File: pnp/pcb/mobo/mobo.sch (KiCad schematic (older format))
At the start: 19 parts, among them J5 Conn_ARM_JTAG_SWD_10, SW2 RESET, U1 STM32F407VETx, Y1 12MHz, Y3 32.768MHz

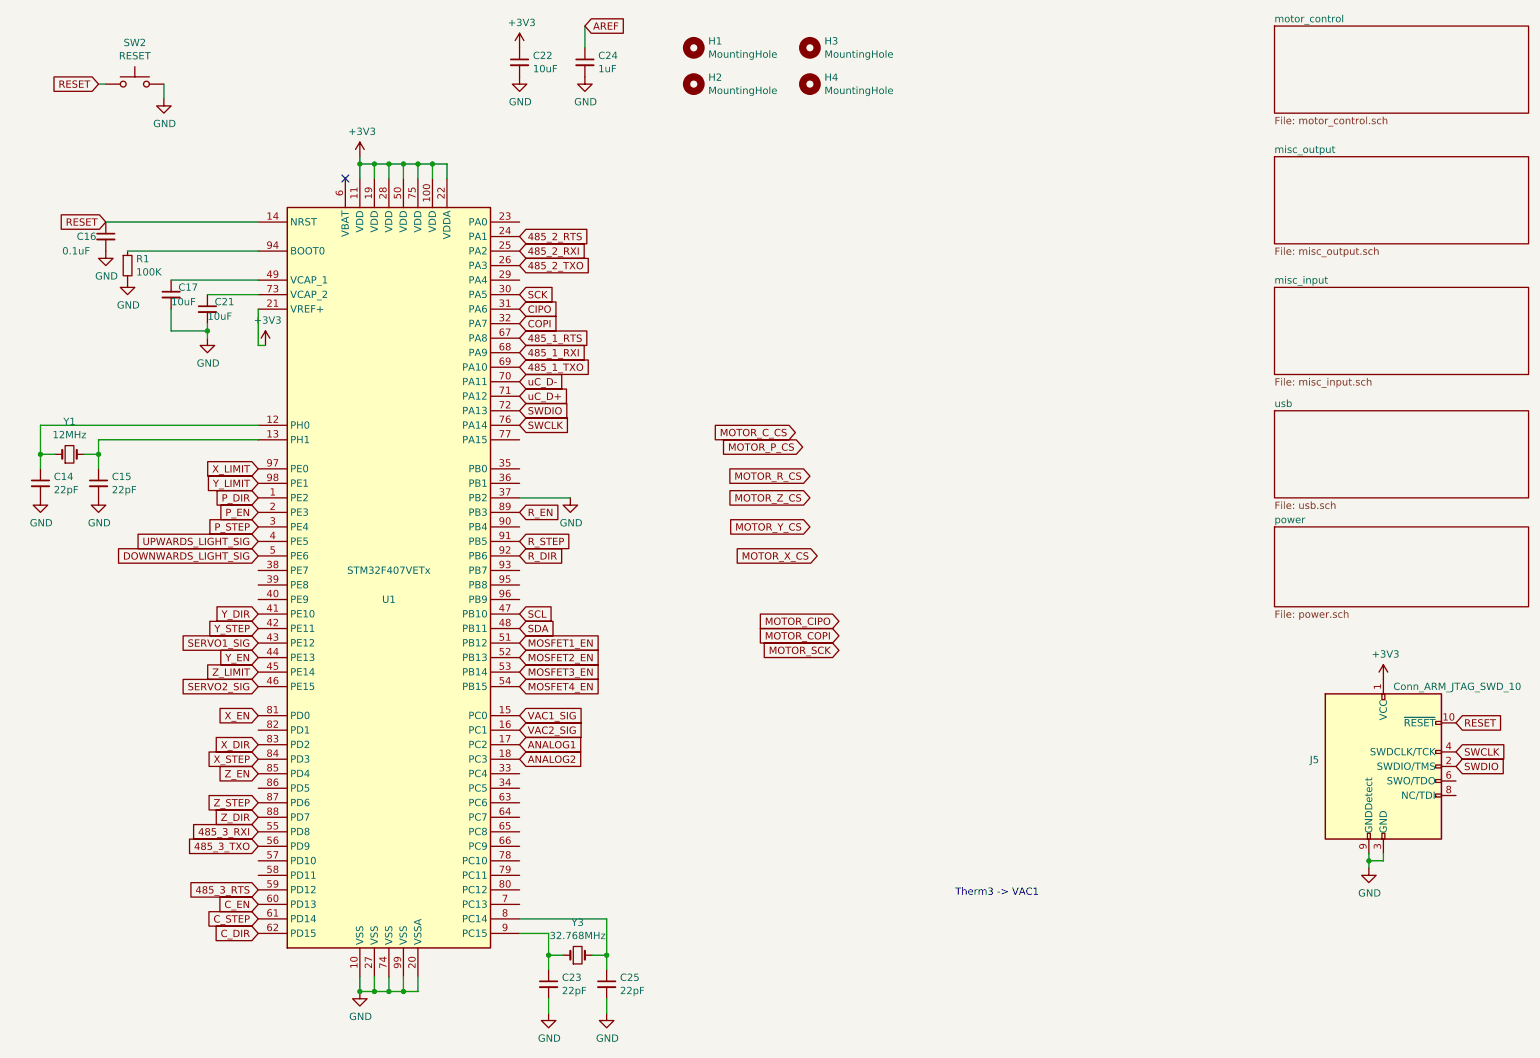
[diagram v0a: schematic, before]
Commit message: finished layout, going to try a different one, committing in case i mess it up
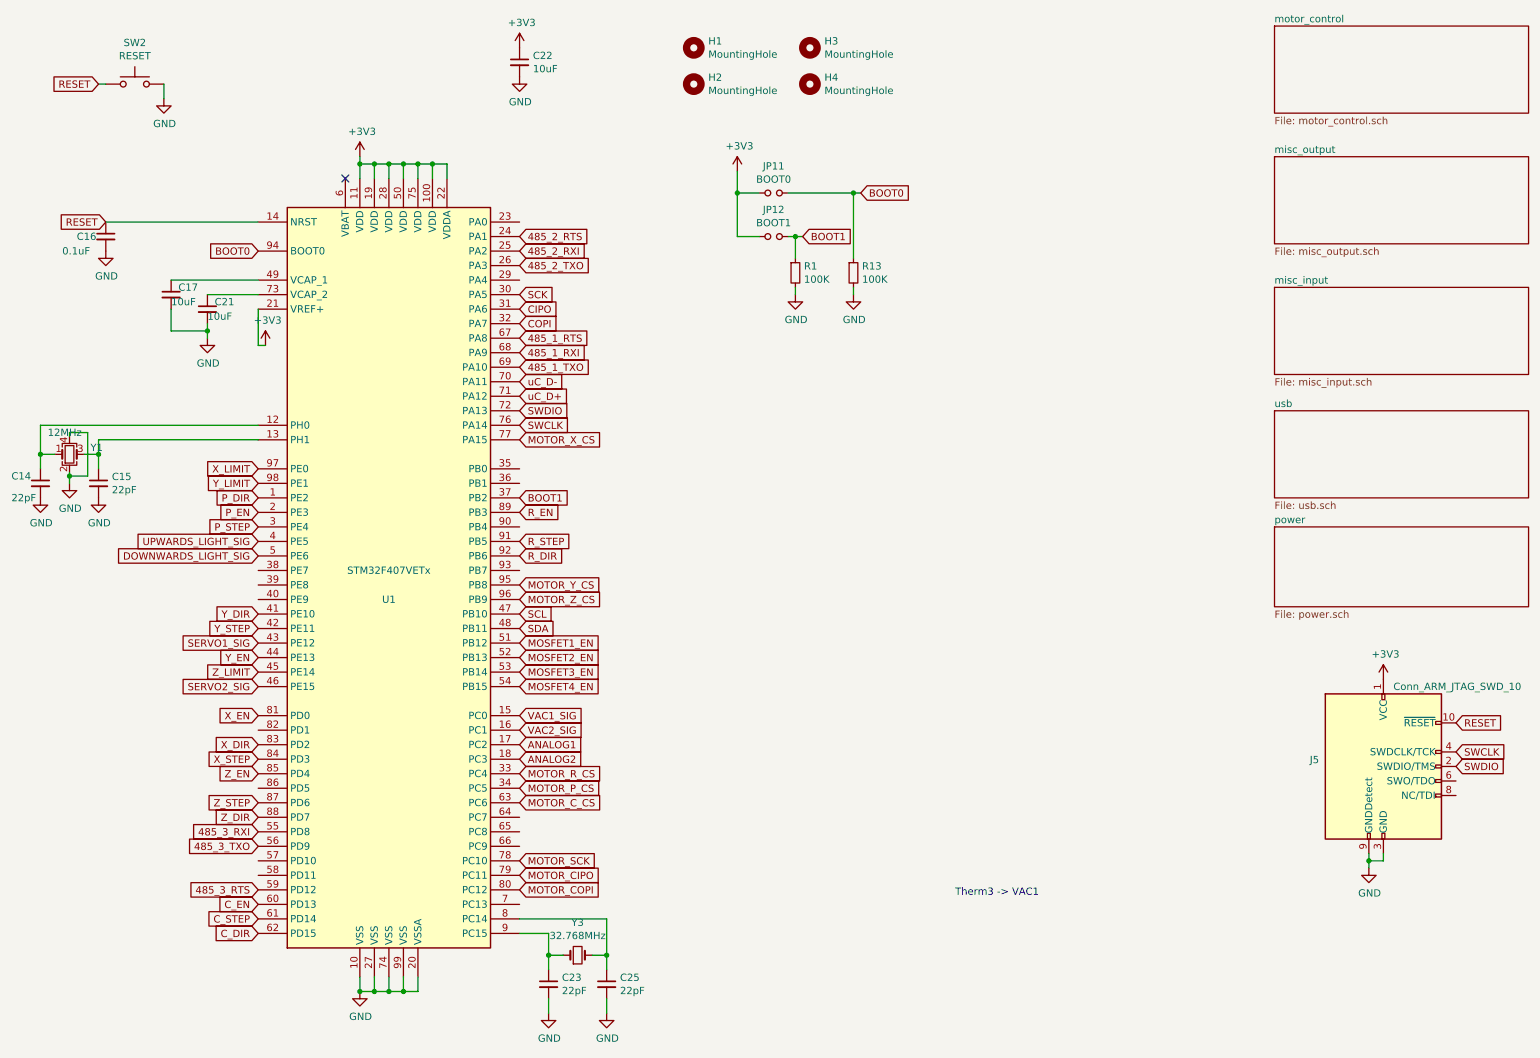
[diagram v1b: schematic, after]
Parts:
- removed C24: 1uF, Capacitor_SMD:C_0805_2012Metric_Pad1.15x1.40mm_HandSolder, symbol Device:C_Small
- removed Y1: 12MHz, Crystal:Crystal_SMD_0603-2Pin_6.0x3.5mm, symbol Device:Crystal_Small
- added JP11: BOOT0, Jumper:SolderJumper-2_P1.3mm_Open_RoundedPad1.0x1.5mm, symbol Device:Jumper_NO_Small
- added JP12: BOOT1, Jumper:SolderJumper-2_P1.3mm_Open_RoundedPad1.0x1.5mm, symbol Device:Jumper_NO_Small
- added R13: 100K, Resistor_SMD:R_0805_2012Metric_Pad1.15x1.40mm_HandSolder, symbol Device:R_Small
- added Y1: 12MHz, Crystal:Crystal_SMD_3225-4Pin_3.2x2.5mm, symbol Device:Crystal_GND24_Small
- Y3: footprint Crystal:Crystal_SMD_0603-2Pin_6.0x3.5mm -> Crystal:Crystal_SMD_3215-2Pin_3.2x1.5mm
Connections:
- net +3V3: now also JP11.1, JP12.1
- net GND: now also R13.2, Y1.2, Y1.4; no longer U1.37 (PB2)
- net MOTOR_CIPO: now also U1.79 (PC11)
- net MOTOR_COPI: now also U1.80 (PC12)
- net MOTOR_C_CS: now also U1.63 (PC6)
- net MOTOR_P_CS: now also U1.34 (PC5)
- net MOTOR_R_CS: now also U1.33 (PC4)
- net MOTOR_SCK: now also U1.78 (PC10)
- net MOTOR_X_CS: now also U1.77 (PA15)
- net MOTOR_Y_CS: now also U1.95 (PB8)
- net MOTOR_Z_CS: now also U1.96 (PB9)
- net at C14.1, U1.12 (PH0): now also Y1.1
- net at C15.1, U1.13 (PH1): now also Y1.3
- net BOOT0: now reaches U1.94 (BOOT0)
- net BOOT0: now also JP11.2, R13.1; no longer R1.1
- new net BOOT1: JP12.2, R1.1, U1.37 (PB2)
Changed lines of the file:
@@
 	1    0    0    -1
 $EndComp
-$Comp
-L Device:C_Small C24
-U 1 1 5EF034CB
-P 4450 900
-F 0 "C24" H 4542 946 50  0000 L CNN
-F 1 "1uF" H 4542 855 50  0000 L CNN
-F 2 "Capacitor_SMD:C_0805_2012Metric_Pad1.15x1.40mm_HandSolder" H 4450 900 50  0001 C CNN
-F 3 "~" H 4450 900 50  0001 C CNN
-	1    4450 900
-	1    0    0    -1
-$EndComp
-$Comp
-L power:GND #PWR0119
-U 1 1 5EF0394F
-P 4450 1000
-F 0 "#PWR0119" H 4450 750 50  0001 C CNN
-F 1 "GND" H 4455 827 50  0000 C CNN
-F 2 "" H 4450 1000 50  0001 C CNN
-F 3 "" H 4450 1000 50  0001 C CNN
-	1    4450 1000
-	1    0    0    -1
-$EndComp
-Text GLabel 4450 650  2    50   Input ~ 0
-AREF
-Wire Wire Line
-	4450 650  4450 800
 Connection ~ 2900 7300
 Wire Wire Line
@@
 $EndComp
 $Comp
-L Device:R_Small R1
-U 1 1 5F0D0BAB
-P 1300 2300
-F 0 "R1" H 1359 2346 50  0000 L CNN
-F 1 "100K" H 1359 2255 50  0000 L CNN
-F 2 "Resistor_SMD:R_0805_2012Metric_Pad1.15x1.40mm_HandSolder" H 1300 2300 50  0001 C CNN
-F 3 "~" H 1300 2300 50  0001 C CNN
-	1    1300 2300
-	1    0    0    -1
-$EndComp
-Wire Wire Line
-	1300 2200 2200 2200
-$Comp
-L power:GND #PWR0121
-U 1 1 5F0D3158
-P 1300 2400
-F 0 "#PWR0121" H 1300 2150 50  0001 C CNN
-F 1 "GND" H 1305 2227 50  0000 C CNN
-F 2 "" H 1300 2400 50  0001 C CNN
-F 3 "" H 1300 2400 50  0001 C CNN
-	1    1300 2400
-	1    0    0    -1
-$EndComp
-$Comp
 L Device:C_Small C17
 U 1 1 5F0D3862
@@
 	1850 2750 1850 2700
 $Comp
-L power:GND #PWR0123
-U 1 1 5F0DF8B3
-P 4350 3900
-F 0 "#PWR0123" H 4350 3650 50  0001 C CNN
-F 1 "GND" H 4355 3727 50  0000 C CNN
-F 2 "" H 4350 3900 50  0001 C CNN
-F 3 "" H 4350 3900 50  0001 C CNN
-	1    4350 3900
-	1    0    0    -1
-$EndComp
-Wire Wire Line
-	4000 3900 4350 3900
-$Comp
-L Device:Crystal_Small Y1
-U 1 1 5F0E1806
-P 900 3600
-F 0 "Y1" H 900 3825 50  0000 C CNN
-F 1 "12MHz" H 900 3734 50  0000 C CNN
-F 2 "Crystal:Crystal_SMD_0603-2Pin_6.0x3.5mm" H 900 3600 50  0001 C CNN
-F 3 "~" H 900 3600 50  0001 C CNN
-	1    900  3600
-	1    0    0    -1
-$EndComp
-$Comp
 L Device:Crystal_Small Y3
 U 1 1 5F0E266F
@@
 F 0 "Y3" H 4400 7275 50  0000 C CNN
 F 1 "32.768MHz" H 4400 7184 50  0000 C CNN
-F 2 "Crystal:Crystal_SMD_0603-2Pin_6.0x3.5mm" H 4400 7050 50  0001 C CNN
+F 2 "Crystal:Crystal_SMD_3215-2Pin_3.2x1.5mm" H 4400 7050 50  0001 C CNN
 F 3 "~" H 4400 7050 50  0001 C CNN
 	1    4400 7050
@@
 U 1 1 5F10974E
 P 700 3800
-F 0 "C14" H 792 3846 50  0000 L CNN
-F 1 "22pF" H 792 3755 50  0000 L CNN
+F 0 "C14" H 500 3850 50  0000 L CNN
+F 1 "22pF" H 500 3700 50  0000 L CNN
 F 2 "Capacitor_SMD:C_0805_2012Metric_Pad1.15x1.40mm_HandSolder" H 700 3800 50  0001 C CNN
 F 3 "~" H 700 3800 50  0001 C CNN
@@
 Text GLabel 2200 6600 0    50   Input ~ 0
 485_3_RTS
-Text GLabel 6200 4750 0    50   Input ~ 0
+Text GLabel 4000 6500 2    50   Input ~ 0
 MOTOR_CIPO
-Text GLabel 6200 4850 0    50   Input ~ 0
+Text GLabel 4000 6600 2    50   Input ~ 0
 MOTOR_COPI
-Text GLabel 6200 4950 0    50   Input ~ 0
+Text GLabel 4000 6400 2    50   Input ~ 0
 MOTOR_SCK
-Text GLabel 6050 4300 0    50   Input ~ 0
+Text GLabel 4000 3500 2    50   Input ~ 0
 MOTOR_X_CS
-Text GLabel 6000 4100 0    50   Input ~ 0
+Text GLabel 4000 4500 2    50   Input ~ 0
 MOTOR_Y_CS
-Text GLabel 6000 3900 0    50   Input ~ 0
+Text GLabel 4000 4600 2    50   Input ~ 0
 MOTOR_Z_CS
-Text GLabel 6000 3750 0    50   Input ~ 0
+Text GLabel 4000 5800 2    50   Input ~ 0
 MOTOR_R_CS
-Text GLabel 5950 3550 0    50   Input ~ 0
+Text GLabel 4000 5900 2    50   Input ~ 0
 MOTOR_P_CS
-Text GLabel 5900 3450 0    50   Input ~ 0
+Text GLabel 4000 6000 2    50   Input ~ 0
 MOTOR_C_CS
+$Comp
+L Device:R_Small R1
+U 1 1 5F1837F8
+P 5900 2350
+F 0 "R1" H 5959 2396 50  0000 L CNN
+F 1 "100K" H 5959 2305 50  0000 L CNN
+F 2 "Resistor_SMD:R_0805_2012Metric_Pad1.15x1.40mm_HandSolder" H 5900 2350 50  0001 C CNN
+F 3 "~" H 5900 2350 50  0001 C CNN
+	1    5900 2350
+	1    0    0    -1
+$EndComp
+Text GLabel 2200 2200 0    50   Input ~ 0
+BOOT0
+Text GLabel 6350 1800 2    50   Input ~ 0
+BOOT0
+Text GLabel 4000 3900 2    50   Input ~ 0
+BOOT1
+Text GLabel 5950 2100 2    50   Input ~ 0
+BOOT1
+$Comp
+L power:+3V3 #PWR0103
+U 1 1 5F186319
+P 5500 1650
+F 0 "#PWR0103" H 5500 1500 50  0001 C CNN
+F 1 "+3V3" H 5515 1823 50  0000 C CNN
+F 2 "" H 5500 1650 50  0001 C CNN
+F 3 "" H 5500 1650 50  0001 C CNN
+	1    5500 1650
+	1    0    0    -1
+$EndComp
+$Comp
+L Device:Jumper_NO_Small JP11
+U 1 1 5F1876E6
+P 5750 1800
+F 0 "JP11" H 5750 1985 50  0000 C CNN
+F 1 "BOOT0" H 5750 1894 50  0000 C CNN
+F 2 "Jumper:SolderJumper-2_P1.3mm_Open_RoundedPad1.0x1.5mm" H 5750 1800 50  0001 C CNN
+F 3 "~" H 5750 1800 50  0001 C CNN
+	1    5750 1800
+	1    0    0    -1
+$EndComp
+$Comp
+L Device:Jumper_NO_Small JP12
+U 1 1 5F1878C4
+P 5750 2100
+F 0 "JP12" H 5750 2285 50  0000 C CNN
+F 1 "BOOT1" H 5750 2194 50  0000 C CNN
+F 2 "Jumper:SolderJumper-2_P1.3mm_Open_RoundedPad1.0x1.5mm" H 5750 2100 50  0001 C CNN
+F 3 "~" H 5750 2100 50  0001 C CNN
+	1    5750 2100
+	1    0    0    -1
+$EndComp
+Wire Wire Line
+	5500 1650 5500 1800
+Wire Wire Line
+	5500 1800 5650 1800
+Wire Wire Line
+	5500 1800 5500 2100
+Wire Wire Line
+	5500 2100 5650 2100
+Connection ~ 5500 1800
+Wire Wire Line
+	5850 1800 6300 1800
+Wire Wire Line
+	5850 2100 5900 2100
+Wire Wire Line
+	5900 2250 5900 2100
+Connection ~ 5900 2100
+Wire Wire Line
+	5900 2100 5950 2100
+$Comp
+L Device:R_Small R13
+U 1 1 5F18E7E3
+P 6300 2350
+F 0 "R13" H 6359 2396 50  0000 L CNN
+F 1 "100K" H 6359 2305 50  0000 L CNN
+F 2 "Resistor_SMD:R_0805_2012Metric_Pad1.15x1.40mm_HandSolder" H 6300 2350 50  0001 C CNN
+F 3 "~" H 6300 2350 50  0001 C CNN
+	1    6300 2350
+	1    0    0    -1
+$EndComp
+Wire Wire Line
+	6300 2250 6300 1800
+Connection ~ 6300 1800
+Wire Wire Line
+	6300 1800 6350 1800
+$Comp
+L power:GND #PWR0105
+U 1 1 5F1902E4
+P 5900 2500
+F 0 "#PWR0105" H 5900 2250 50  0001 C CNN
+F 1 "GND" H 5905 2327 50  0000 C CNN
+F 2 "" H 5900 2500 50  0001 C CNN
+F 3 "" H 5900 2500 50  0001 C CNN
+	1    5900 2500
+	1    0    0    -1
+$EndComp
+$Comp
+L power:GND #PWR0107
+U 1 1 5F19074C
+P 6300 2500
+F 0 "#PWR0107" H 6300 2250 50  0001 C CNN
+F 1 "GND" H 6305 2327 50  0000 C CNN
+F 2 "" H 6300 2500 50  0001 C CNN
+F 3 "" H 6300 2500 50  0001 C CNN
+	1    6300 2500
+	1    0    0    -1
+$EndComp
+Wire Wire Line
+	6300 2500 6300 2450
+Wire Wire Line
+	5900 2500 5900 2450
+$Comp
+L Device:Crystal_GND24_Small Y1
+U 1 1 5F20EB5B
+P 900 3600
+F 0 "Y1" H 1044 3646 50  0000 L CNN
+F 1 "12MHz" H 750 3750 50  0000 L CNN
+F 2 "Crystal:Crystal_SMD_3225-4Pin_3.2x2.5mm" H 900 3600 50  0001 C CNN
+F 3 "~" H 900 3600 50  0001 C CNN
+	1    900  3600
+	1    0    0    -1
+$EndComp
+$Comp
+L power:GND #PWR0119
+U 1 1 5F2115D3
+P 900 3800
+F 0 "#PWR0119" H 900 3550 50  0001 C CNN
+F 1 "GND" H 905 3627 50  0000 C CNN
+F 2 "" H 900 3800 50  0001 C CNN
+F 3 "" H 900 3800 50  0001 C CNN
+	1    900  3800
+	1    0    0    -1
+$EndComp
+Wire Wire Line
+	900  3725 900  3750
+Wire Wire Line
+	900  3475 900  3450
+Wire Wire Line
+	900  3450 1025 3450
+Wire Wire Line
+	1025 3450 1025 3750
+Wire Wire Line
+	1025 3750 900  3750
+Connection ~ 900  3750
+Wire Wire Line
+	900  3750 900  3800
 $EndSCHEMATC
